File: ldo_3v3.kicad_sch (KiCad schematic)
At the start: 4 parts, among them U3701 SE8633K2-HF

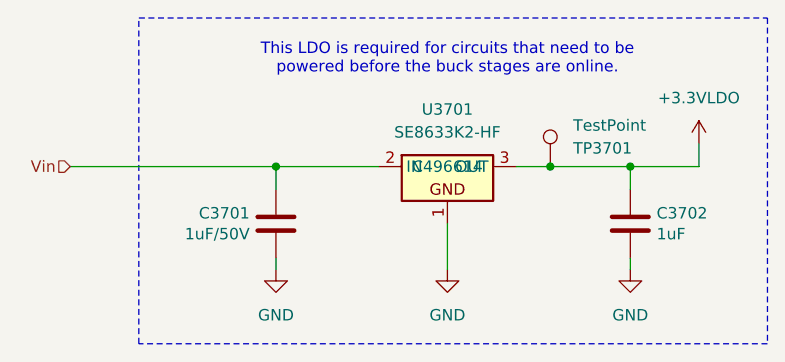
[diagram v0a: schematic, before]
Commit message: Further refinements
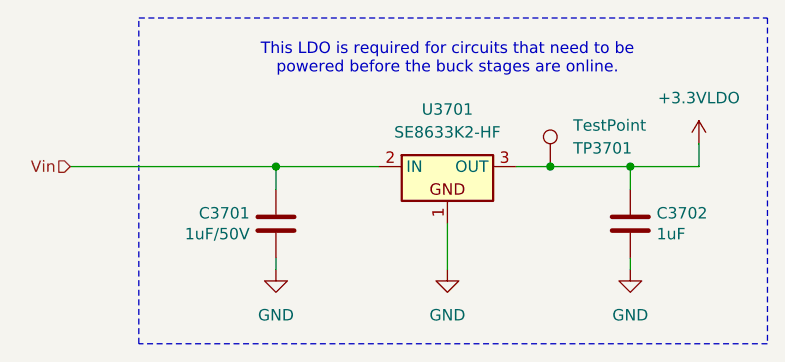
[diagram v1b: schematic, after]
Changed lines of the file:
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@@
+			)
+		)
+		(property "LCSC Part" ""
+			(at 157.48 96.52 0)
+			(effects
+				(font
+					(size 1.27 1.27)
+				)
+			)
+		)
+		(property "Sim.Enable" ""
+			(at 157.48 96.52 0)
+			(effects
+				(font
+					(size 1.27 1.27)
+				)
 			)
 		)
@@
 			)
 		)
+		(property "LCSC Part" ""
+			(at 166.37 102.87 0)
+			(effects
+				(font
+					(size 1.27 1.27)
+				)
+			)
+		)
+		(property "Sim.Enable" ""
+			(at 166.37 102.87 0)
+			(effects
+				(font
+					(size 1.27 1.27)
+				)
+			)
+		)
 		(pin "1"
 		)
@@
 					(size 1.27 1.27)
 				)
+				(hide yes)
+			)
+		)
+		(property "Sim.Enable" ""
+			(at 146.05 96.52 0)
+			(effects
+				(font
+					(size 1.27 1.27)
+				)
 			)
 		)
@@
 			)
 		)
+		(property "LCSC Part" ""
+			(at 127 102.87 0)
+			(effects
+				(font
+					(size 1.27 1.27)
+				)
+			)
+		)
+		(property "Sim.Enable" ""
+			(at 127 102.87 0)
+			(effects
+				(font
+					(size 1.27 1.27)
+				)
+			)
+		)
